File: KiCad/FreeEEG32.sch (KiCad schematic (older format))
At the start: 30 parts, among them P11 CONN_01X03, SW1 NRST, U1 ADP7118AUJZ-3.3_TSOT, U2 ADP7118AUJZ-3.3_TSOT, U3 8.192MHz, U37 STM32F427ZI_4side_short, U39 ADP7118AUJZ-3.3_TSOT, U4 STM32F427ZI_4side, U43 473521001, Y1 32.768kHz, Y2 8MHz

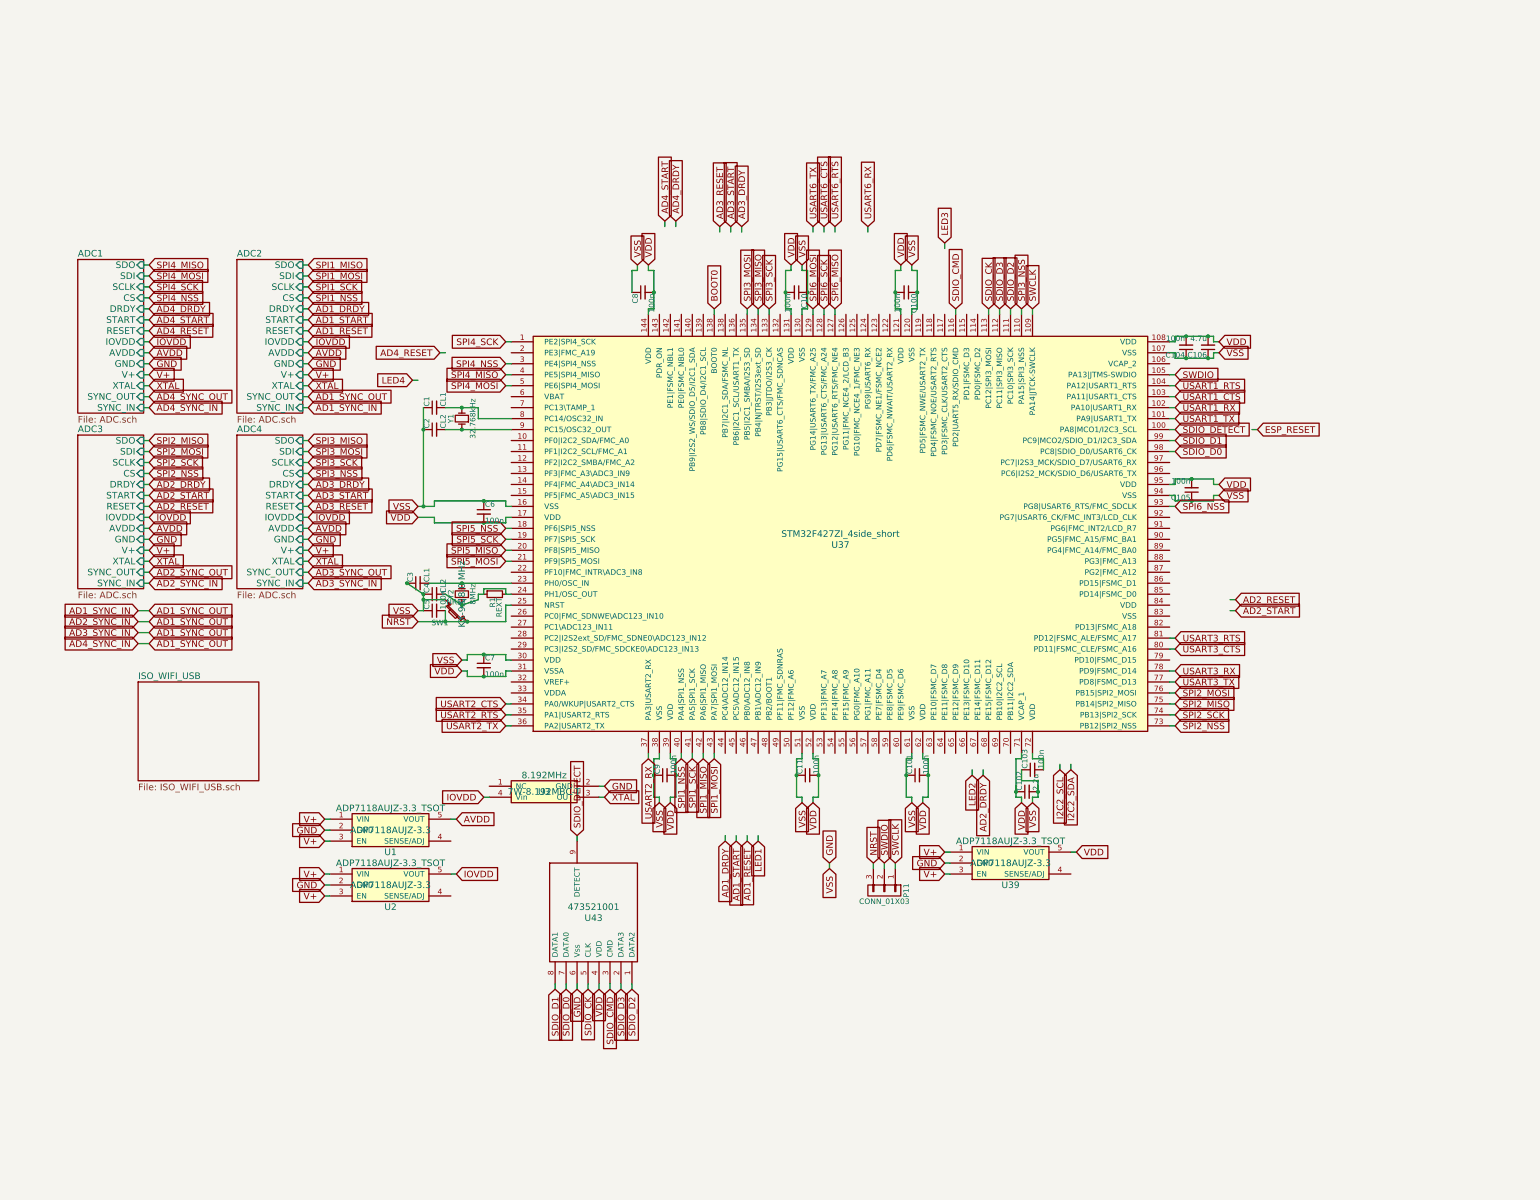
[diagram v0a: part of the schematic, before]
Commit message: kicad
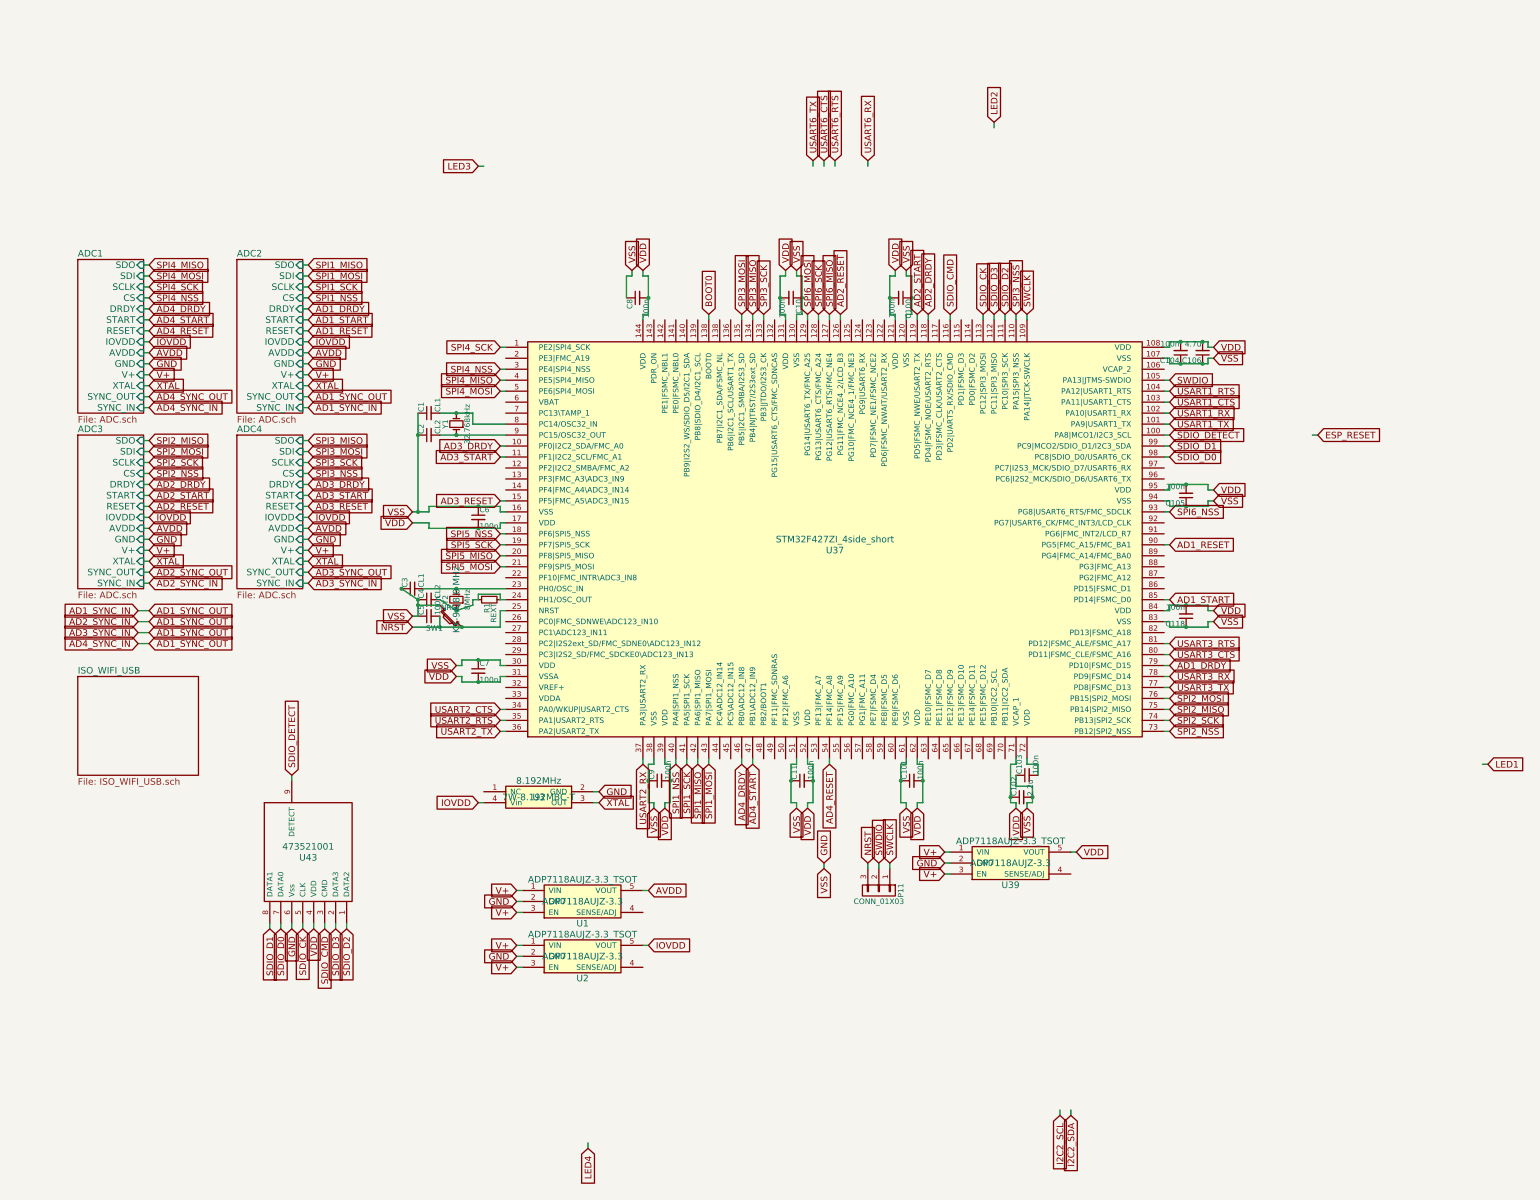
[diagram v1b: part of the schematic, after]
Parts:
- added C118: 100n, Capacitors_SMD:C_0402, symbol C_Small
- Y2: footprint Crystals:Crystal_SMD_5032-4pin_5.0x3.2mm -> Crystals:Crystal_SMD_5032_4Pads
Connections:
- wire segments 292 -> 302
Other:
- moved on the sheet: C1, C10, C100, C101, C102, C103, C104, C105, C106, C11, C2, C3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
